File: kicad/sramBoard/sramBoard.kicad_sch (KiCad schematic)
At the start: 0 parts

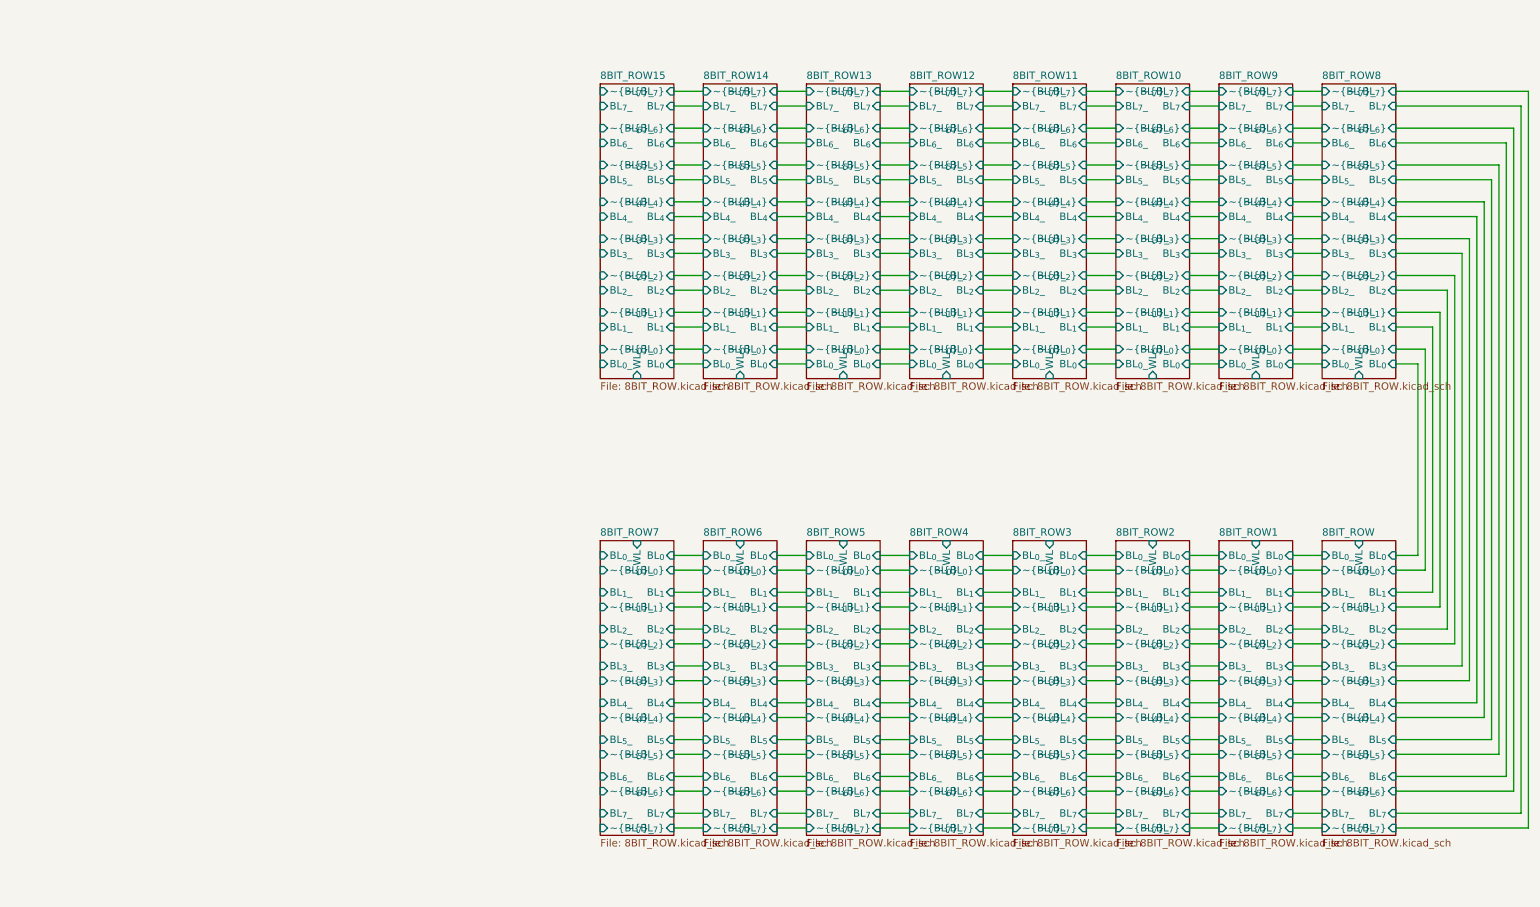
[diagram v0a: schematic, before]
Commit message: Initial ram board schematic
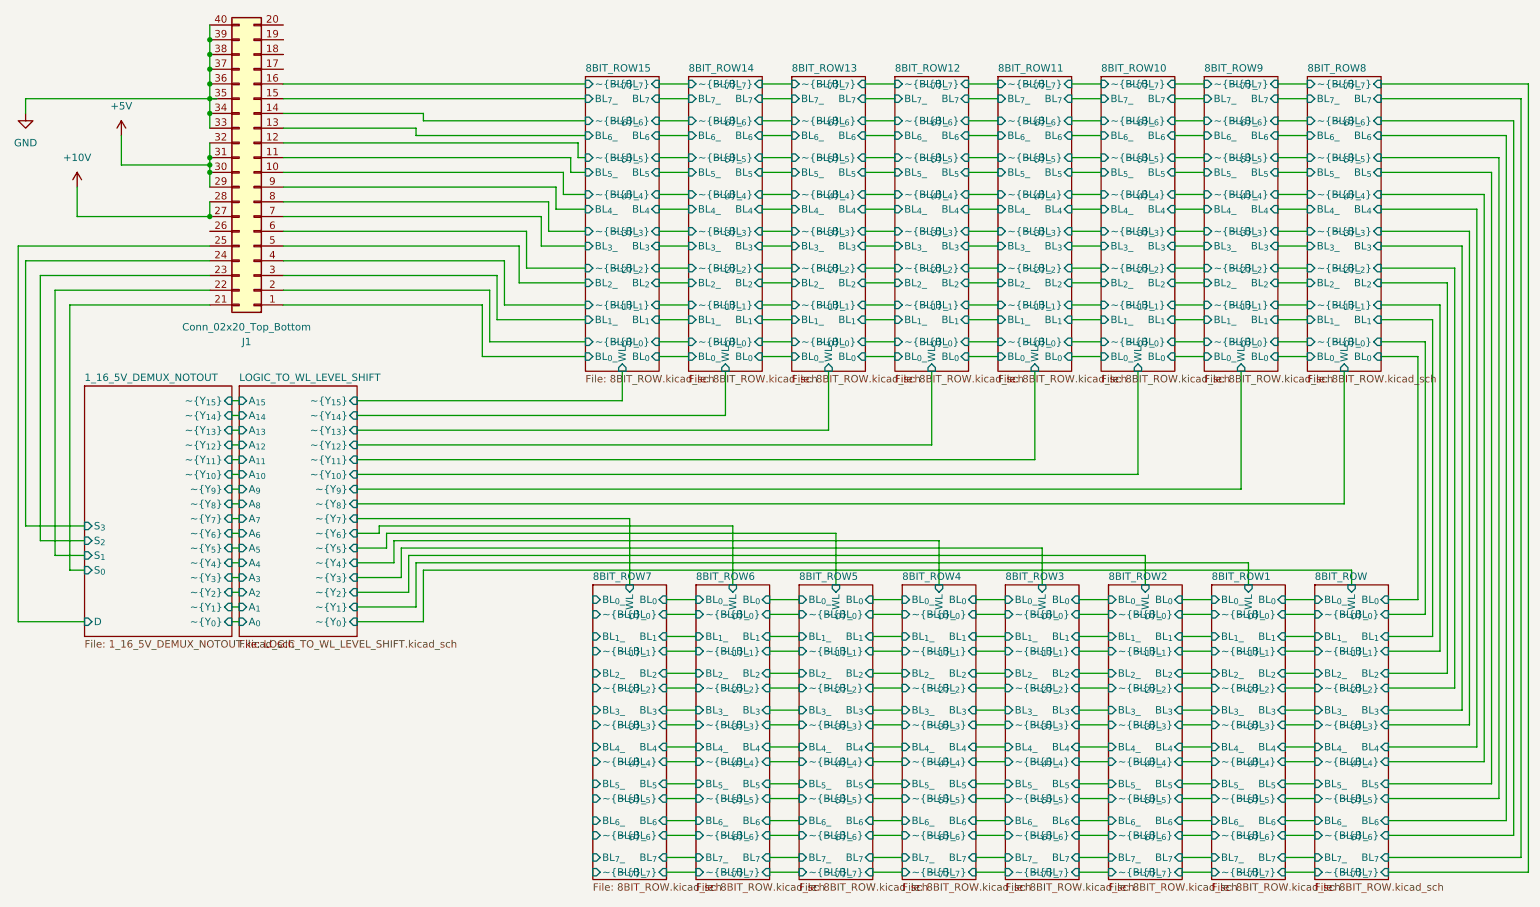
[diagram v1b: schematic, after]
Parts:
- added J1: Conn_02x20_Top_Bottom, symbol Connector_Generic:Conn_02x20_Top_Bottom
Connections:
- net 8BIT_ROW15/BL_{0}_: now also J1.1 (Pin_1)
- net 8BIT_ROW15/BL_{1}_: now also J1.3 (Pin_3)
- net 8BIT_ROW15/BL_{2}_: now also J1.5 (Pin_5)
- net 8BIT_ROW15/BL_{3}_: now also J1.7 (Pin_7)
- net 8BIT_ROW15/BL_{4}_: now also J1.9 (Pin_9)
- net 8BIT_ROW15/BL_{5}_: now also J1.11 (Pin_11)
- net 8BIT_ROW15/BL_{6}_: now also J1.13 (Pin_13)
- net 8BIT_ROW15/BL_{7}_: now also J1.15 (Pin_15)
- net 8BIT_ROW15/~{BL_{0}}_: now also J1.2 (Pin_2)
- net 8BIT_ROW15/~{BL_{1}}_: now also J1.4 (Pin_4)
- net 8BIT_ROW15/~{BL_{2}}_: now also J1.6 (Pin_6)
- net 8BIT_ROW15/~{BL_{3}}_: now also J1.8 (Pin_8)
- net 8BIT_ROW15/~{BL_{4}}_: now also J1.10 (Pin_10)
- net 8BIT_ROW15/~{BL_{5}}_: now also J1.12 (Pin_12)
- net 8BIT_ROW15/~{BL_{6}}_: now also J1.14 (Pin_14)
- net 8BIT_ROW15/~{BL_{7}}_: now also J1.16 (Pin_16)
- new net +10V: J1.27 (Pin_27), J1.28 (Pin_28)
- new net +5V: J1.29 (Pin_29), J1.30 (Pin_30), J1.31 (Pin_31), J1.32 (Pin_32)
- new net 1_16_5V_DEMUX_NOTOUT/D: J1.25 (Pin_25)
- new net 1_16_5V_DEMUX_NOTOUT/S_{0}: J1.21 (Pin_21)
- new net 1_16_5V_DEMUX_NOTOUT/S_{1}: J1.22 (Pin_22)
- new net 1_16_5V_DEMUX_NOTOUT/S_{2}: J1.23 (Pin_23)
- new net 1_16_5V_DEMUX_NOTOUT/S_{3}: J1.24 (Pin_24)
- new net GND: J1.33 (Pin_33), J1.34 (Pin_34), J1.35 (Pin_35), J1.36 (Pin_36), J1.37 (Pin_37), J1.38 (Pin_38), J1.39 (Pin_39), J1.40 (Pin_40)
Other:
- added sheet 1_16_5V_DEMUX_NOTOUT (1_16_5V_DEMUX_NOTOUT.kicad_sch)
- added sheet LOGIC_TO_WL_LEVEL_SHIFT (LOGIC_TO_WL_LEVEL_SHIFT.kicad_sch)
